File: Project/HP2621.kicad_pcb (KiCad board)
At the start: 2 copper layers, 300 x 114.3 mm, 185 parts, among them J1 JST SH, J2 Pico EZmate, SW1 RotaryEncoder_Switch, SW2 RotaryEncoder_Switch, SW3 RotaryEncoder_Switch, SW4 RotaryEncoder_Switch, SW5 SKQGABE010, U1 XC6206PxxxMR-Regulator_Linear, U2 STM32F072CBT6

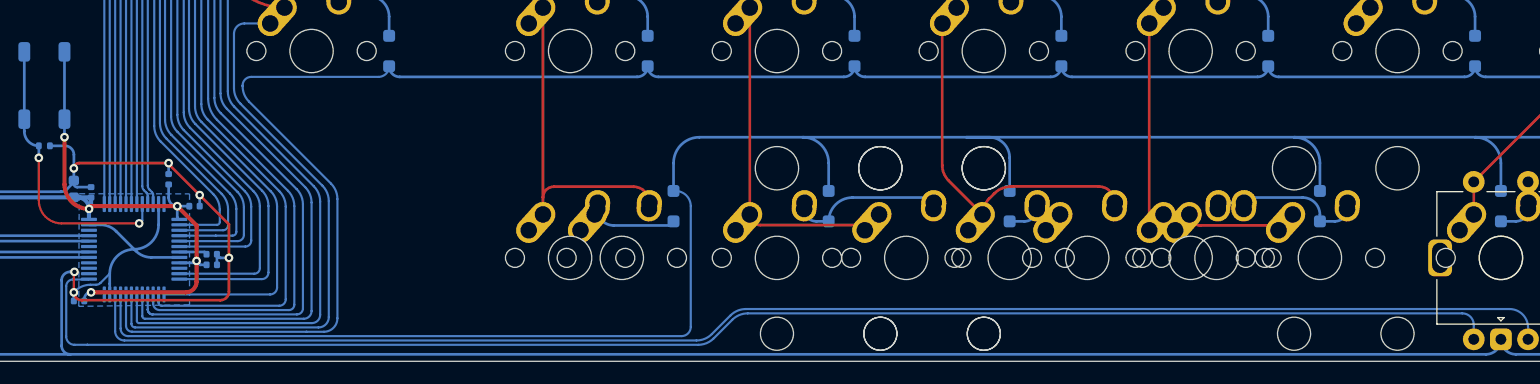
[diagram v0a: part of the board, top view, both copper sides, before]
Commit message: fresh gerbers
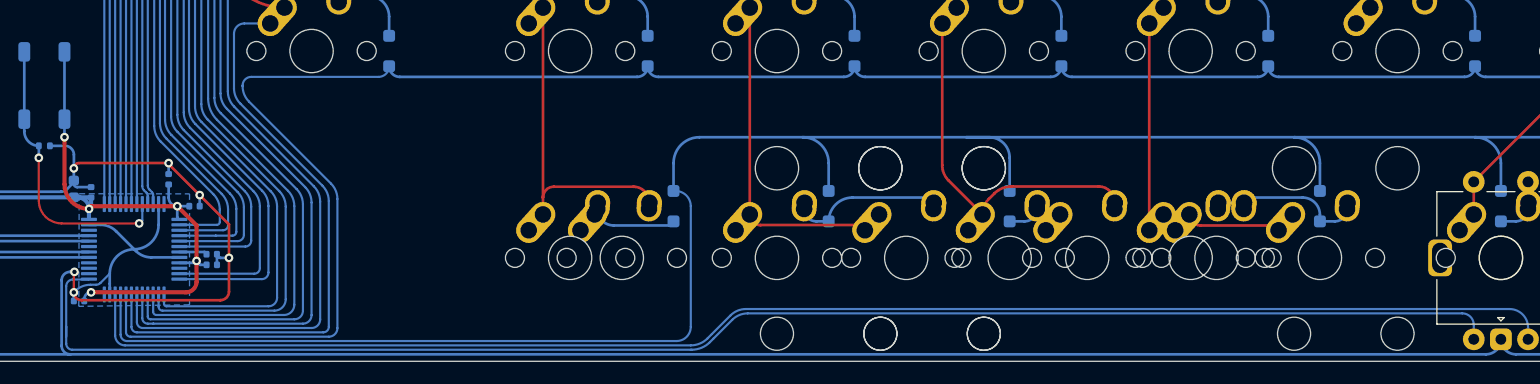
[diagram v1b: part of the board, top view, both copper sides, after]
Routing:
- net COL7: track 270.2 -> 272.2 mm
- net ENC_g: track 140.0 -> 141.6 mm
- net ROW4: track 318.8 -> 320.0 mm
- net COL1: track 126.5 -> 127.5 mm
- net COL4: track 227.8 -> 228.6 mm
- net COL5: track 264.5 -> 265.4 mm
- net COL3: track 231.3 -> 232.0 mm
- net ROW5: track 290.0 -> 290.7 mm
- net COL2: track 207.3 -> 208.0 mm
- net COL6: track 230.5 -> 231.1 mm
- net ENC_h: track 137.0 -> 137.6 mm
